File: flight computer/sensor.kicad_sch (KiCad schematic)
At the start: 163 parts, among them IC1 A3909, J1 Micro_SD_Card_Det1, J12 Conn_01x04, J13 1x3 servo, J14 1x3 servo, J15 arming terminal, J16 arming terminal, J17 arming terminal, J18 arming terminal, J19 Screw_Terminal_01x02, J20 Screw_Terminal_01x02, J21 Screw_Terminal_01x02, J22 Screw_Terminal_01x02, J25 Conn_Coaxial, J3 Conn_Coaxial, J4 H9161TR-ND, J5 Screw_Term, J6 1x3 servo, J9 1x3 servo, Q1 IRLML6402, Q10 IRLML6402, Q11 IRLML6402, Q3 IRLML6402, Q4 IRLML6402, Q5 IRLML6402, Q6 IRLML6402, Q7 BSS138, Q8 IRLML6402, Q9 IRLML6402, U10 LSM6DS3, U11 BGM220SC12WGA2R, U12 PE4259, U2 IMU, U5 LPS22HB, U6 GPS, U7 SX1276, U8 NAND, Y2 32.768kHz, Y4 32MHz

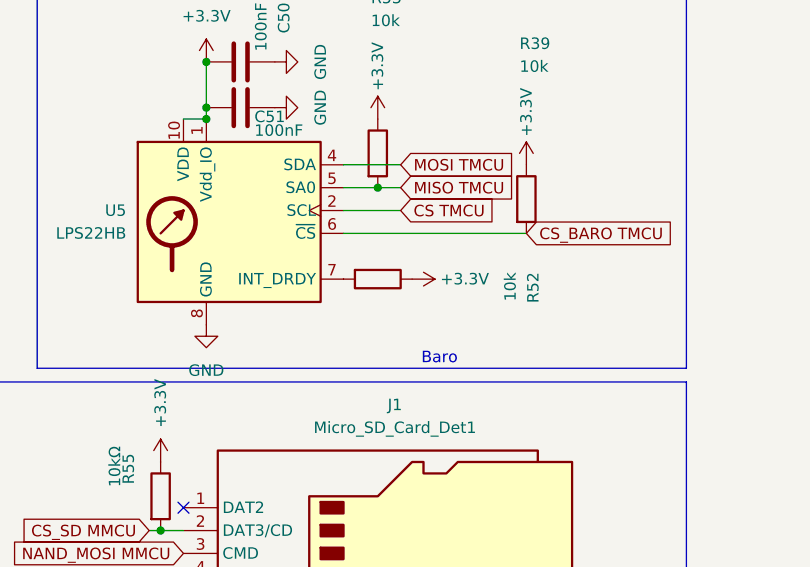
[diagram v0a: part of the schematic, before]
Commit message: Ummm, more baro routing to the MCU and stuff
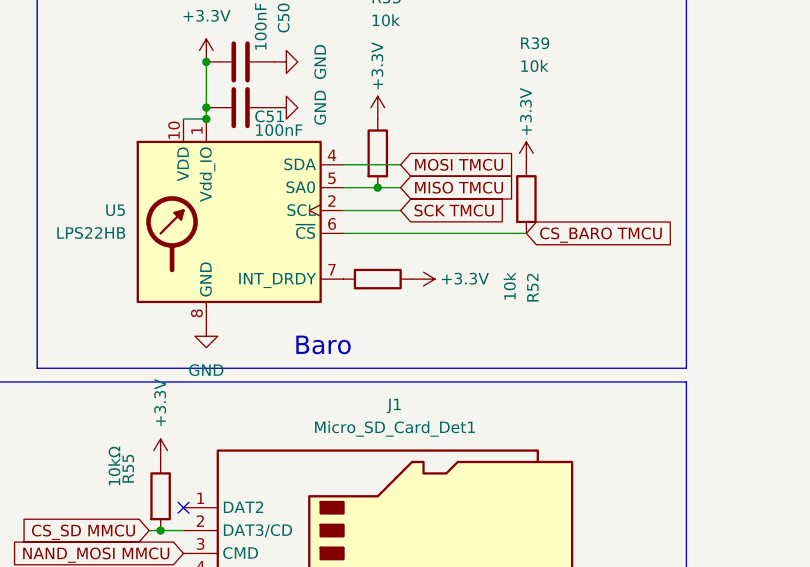
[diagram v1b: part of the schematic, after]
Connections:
- net  SPI0_SCK MMCU is gone; now on net SPI0_SCK MMCU: U8.6 (CLK)
- net CS TMCU renamed SCK TMCU
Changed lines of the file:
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@@
 	(text "Baro"
 		(exclude_from_sim no)
-		(at 255.778 116.84 0)
+		(at 242.824 115.57 0)
 		(effects
 			(font
-				(size 1.27 1.27)
+				(size 2.032 2.032)
 			)
 		)
@@
 		)
 	)
-	(global_label " SPI0_SCK MMCU"
+	(global_label "SPI0_SCK MMCU"
 		(shape input)
 		(at 175.26 137.16 180)
@@
 		)
 		(property "Intersheetrefs" "${INTERSHEET_REFS}"
-			(at 155.8254 137.16 0)
+			(at 156.793 137.16 0)
 			(effects
 				(font
@@
 		)
 	)
-	(global_label "CS TMCU"
+	(global_label "SCK TMCU"
 		(shape input)
 		(at 251.46 100.33 0)
@@
 		)
 		(property "Intersheetrefs" "${INTERSHEET_REFS}"
-			(at 262.9118 100.33 0)
+			(at 264.1818 100.33 0)
 			(effects
 				(font
